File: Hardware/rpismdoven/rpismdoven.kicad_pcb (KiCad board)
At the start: 2 copper layers, 65 x 56.5 mm, 33 parts, among them J1 Raspberry_Pi_2_3, J2 Conn_01x02_Female, J3 T-PROBE, J4 MAX31855-BREAKOUT, Q1 2N2219, Q2 2N2219, U1 MAX31855TASA

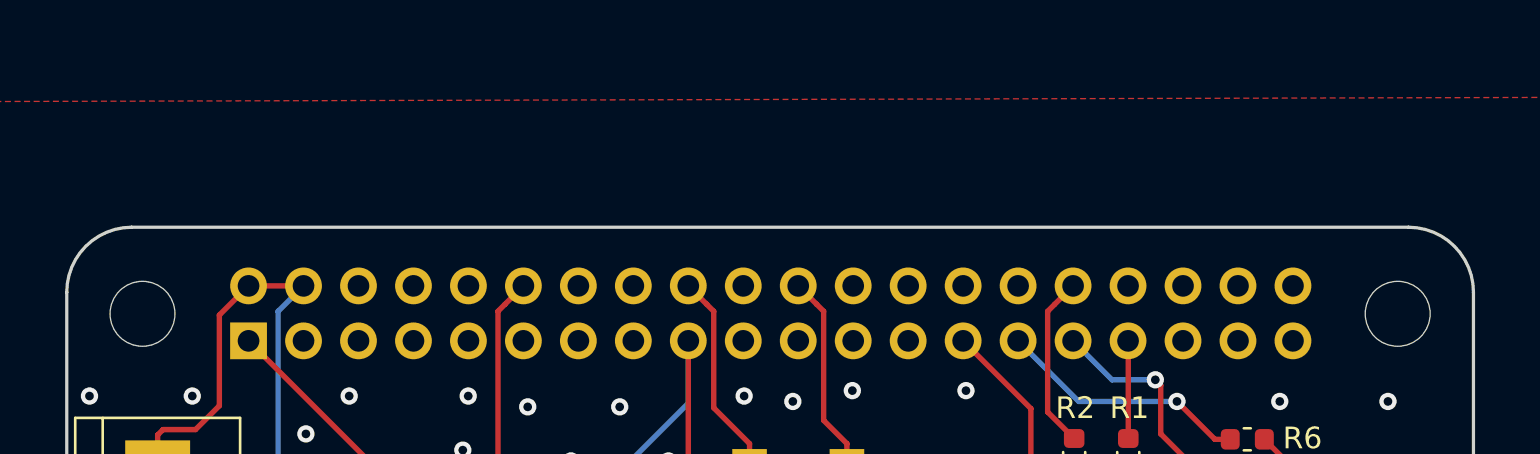
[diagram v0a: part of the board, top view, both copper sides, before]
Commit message: Sorry future me
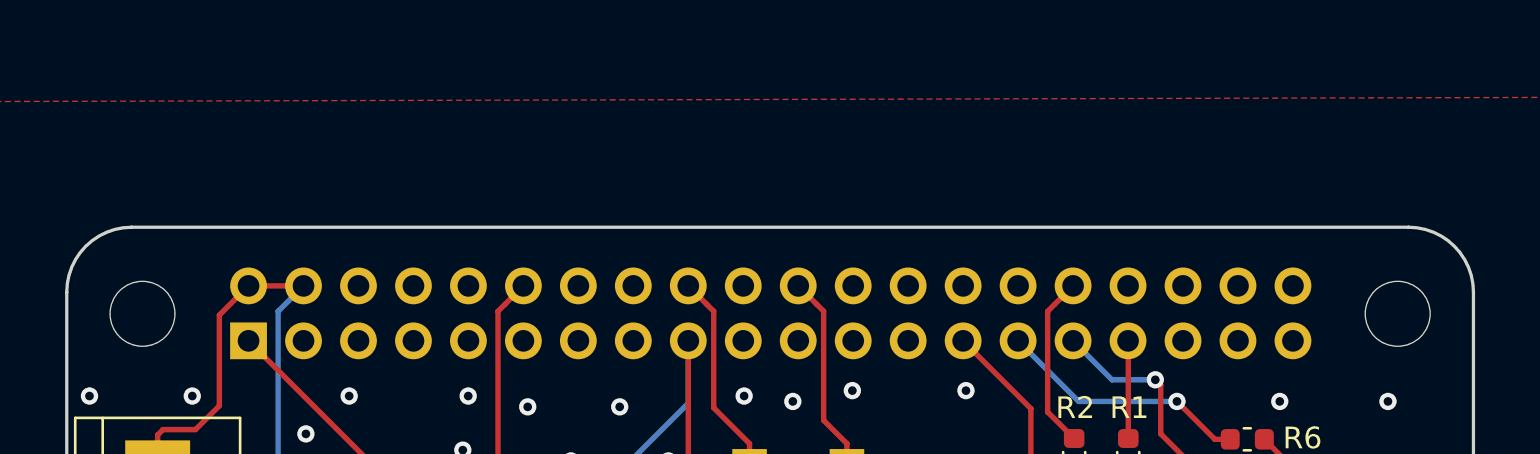
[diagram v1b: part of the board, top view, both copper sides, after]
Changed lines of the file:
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@@
-(kicad_pcb (version 20171130) (host pcbnew "(5.0.0)")
+(kicad_pcb (version 20171130) (host pcbnew "(5.1.0)-1")
   (general
     (thickness 1.6)
@@
     (zone_45_only no)
     (trace_min 0.2)
-    (segment_width 0.2)
-    (edge_width 0.15)
     (via_size 0.8)
     (via_drill 0.4)
@@
     (uvia_min_size 0.2)
     (uvia_min_drill 0.1)
+    (edge_width 0.15)
+    (segment_width 0.2)
     (pcb_text_width 0.3)
     (pcb_text_size 1.5 1.5)
@@
   (gr_arc (start 160.7 57.95) (end 163.7 57.95) (angle -90) (layer Edge.Cuts) (width 0.15))
   (gr_line (start 163.7 108.45) (end 163.7 57.95) (layer Edge.Cuts) (width 0.15))
-  (gr_line (start 160.7 54.95) (end 101.69 54.95) (layer Edge.Cuts) (width 0.15))
+  (gr_line (start 160.7 54.95) (end 101.7 54.95) (layer Edge.Cuts) (width 0.15))
   (segment (start 107.1 57.66) (end 105.75 59.01) (width 0.25) (layer F.Cu) (net 1))
   (segment (start 105.75 59.01) (end 105.75 63.2) (width 0.25) (layer F.Cu) (net 1))
